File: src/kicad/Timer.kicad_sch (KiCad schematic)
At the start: 47 parts, among them J1 Conn_01x02, Q2 Q_NPN_BCE, SW10 SW_DIP_x01, SW2 SW_Push, SW3 SW_SP4T_NR01104, SW4 SW_DIP_x01, SW5 SW_DIP_x01, SW6 SW_DIP_x01, SW7 SW_DIP_x01, SW8 SW_DIP_x01, SW9 SW_DIP_x01, U1 4060, U2 NE555P, U3 NE555P

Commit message: Add files via upload
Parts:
- U1: footprint Package_SO:SOIC-16W_5.3x10.2mm_P1.27mm -> Package_DIP:DIP-16_W7.62mm
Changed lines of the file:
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@@
 			)
 		)
-		(property "Footprint" "Package_SO:SOIC-16W_5.3x10.2mm_P1.27mm"
+		(property "Footprint" "Package_DIP:DIP-16_W7.62mm"
 			(at 71.12 80.01 0)
 			(hide yes)

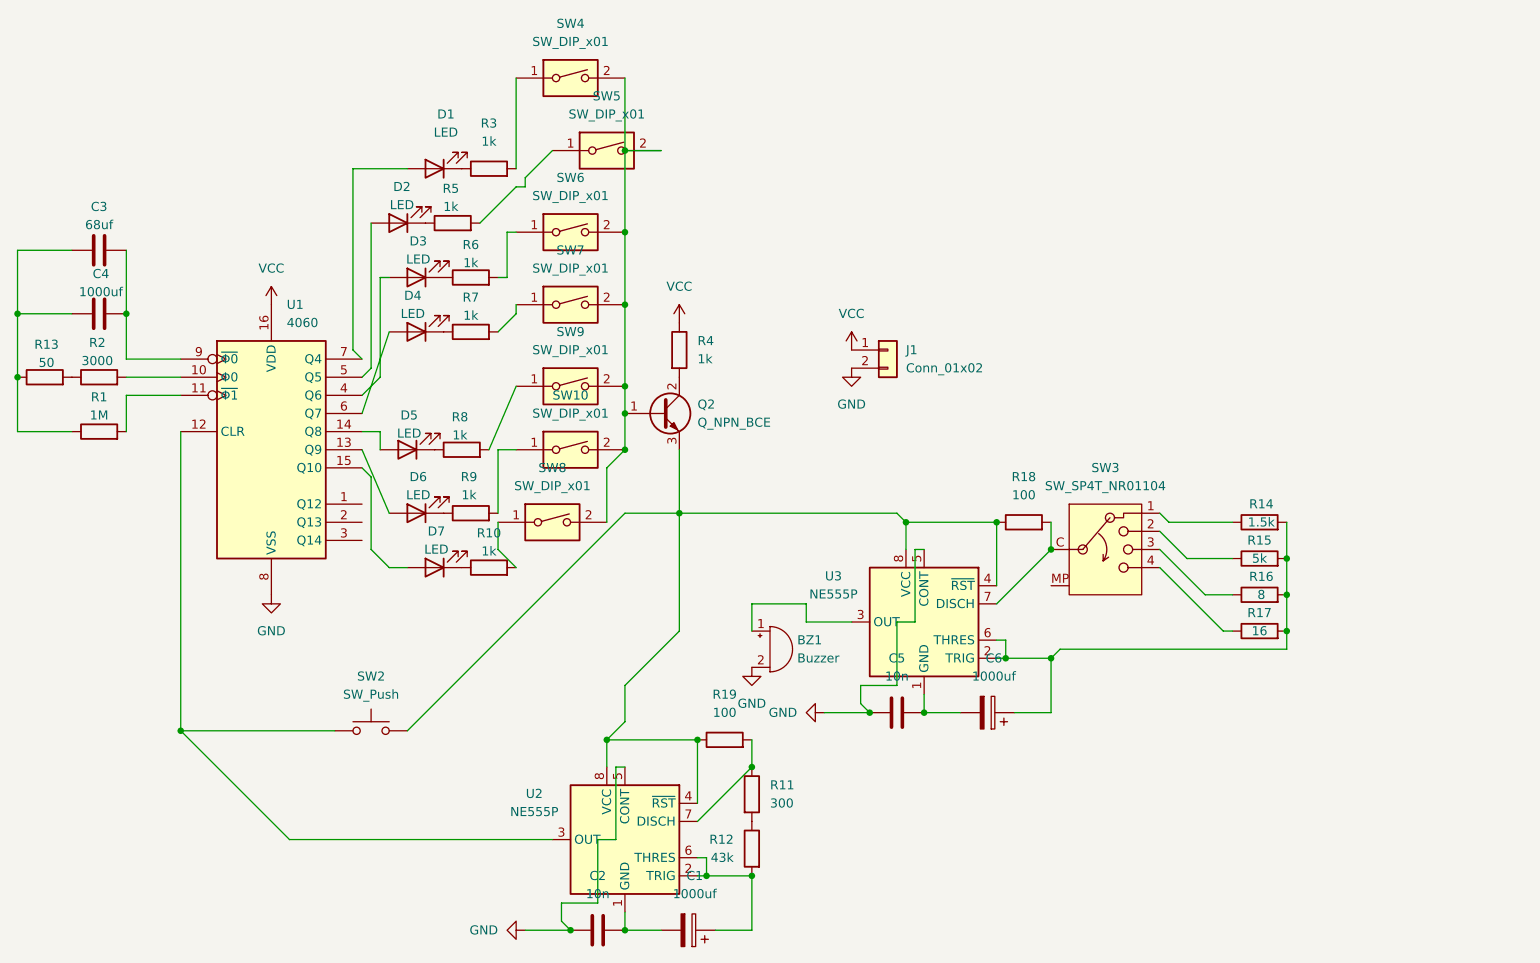
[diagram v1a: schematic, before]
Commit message: Add files via upload
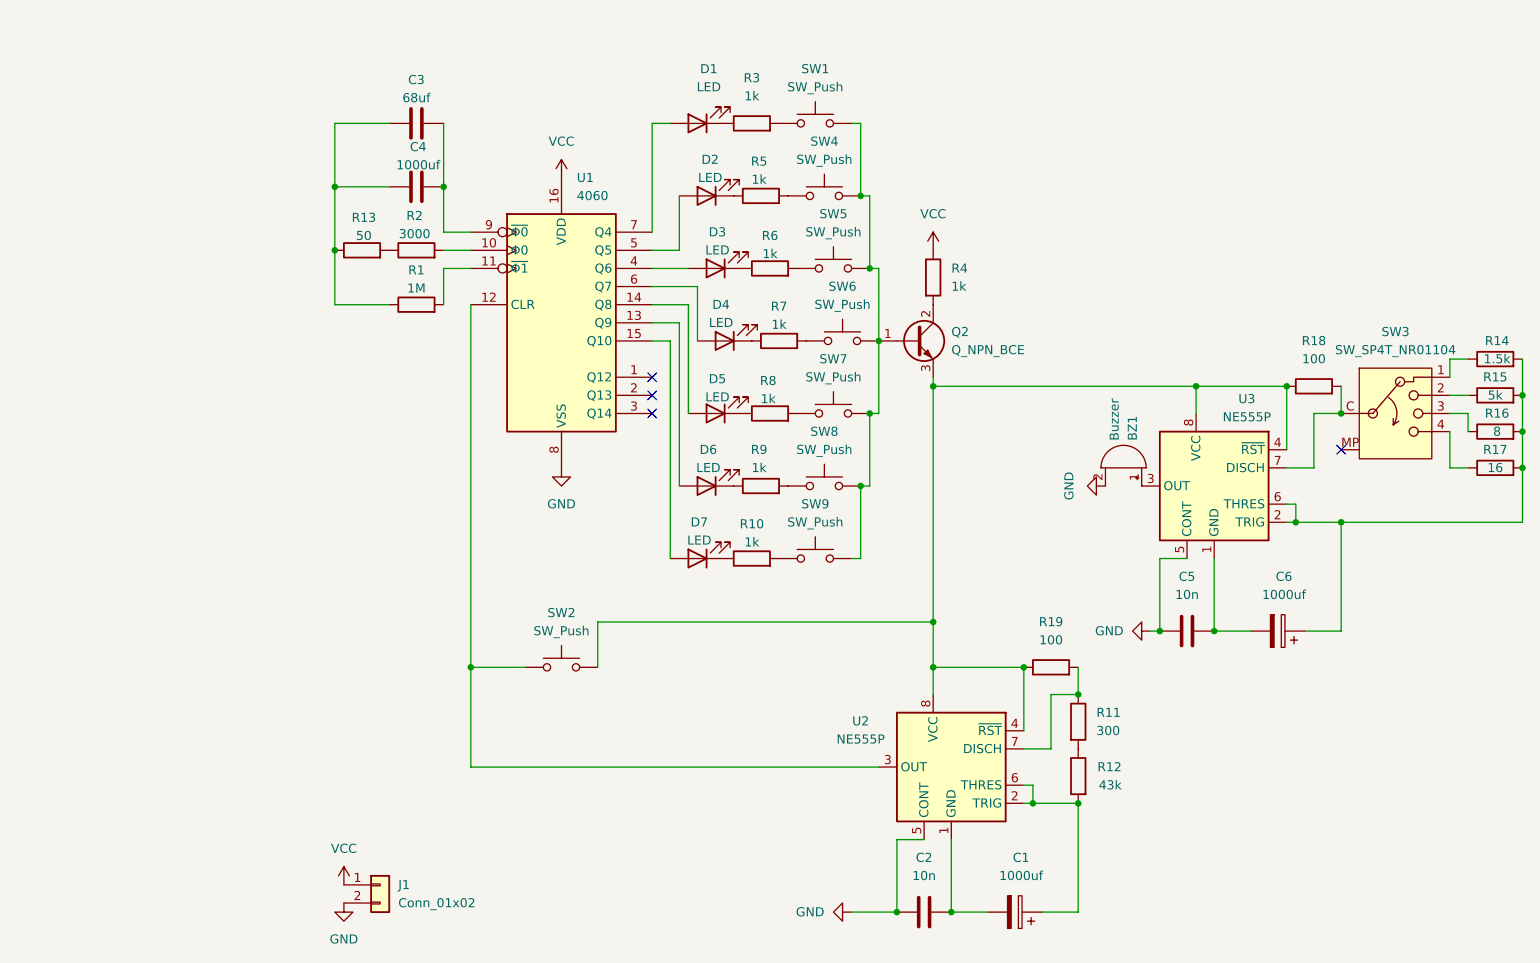
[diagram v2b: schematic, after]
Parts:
- removed SW10, SW4, SW5, SW6, SW7, SW8, SW9: SW_DIP_x01, Button_Switch_THT:SW_PUSH_6mm, symbol Switch:SW_DIP_x01
- added SW1, SW4, SW5, SW6, SW7, SW8, SW9: SW_Push, Button_Switch_THT:SW_PUSH_6mm, symbol Switch:SW_Push
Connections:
- net at R8.2: now also SW7.1
- net at R9.2: now also SW8.1
- net at R7.2: now also SW6.1
- net at Q2.1 (B): now also SW1.2, SW4.2, SW5.2, SW6.2, SW7.2, SW8.2, SW9.2
- net at R3.2: now also SW1.1
- net at R6.2: now also SW5.1
- net at R10.2: now also SW9.1
- net at R5.2: now also SW4.1
- no-connect marks 0 -> 4
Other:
- moved on the sheet: BZ1, C1, C2, C3, C4, C5, C6, D1, D2, D3, D4, D5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
